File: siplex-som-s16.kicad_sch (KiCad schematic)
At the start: 1 part, among them J1 RFShield_OnePiece

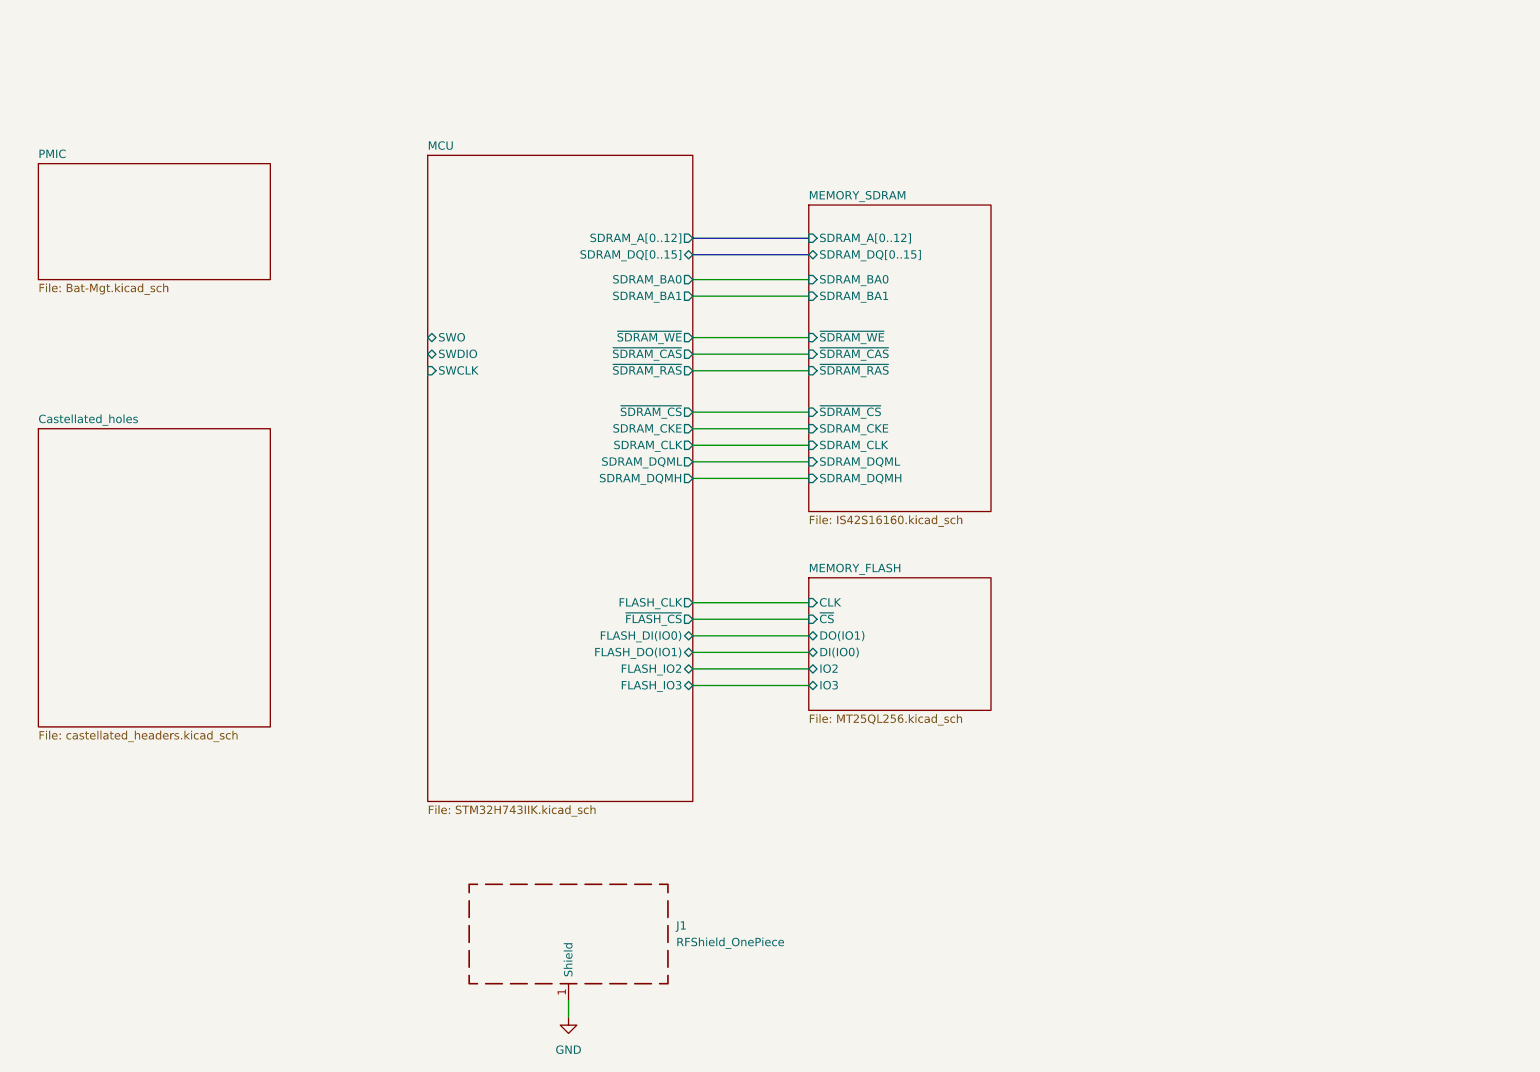
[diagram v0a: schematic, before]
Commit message: Add power
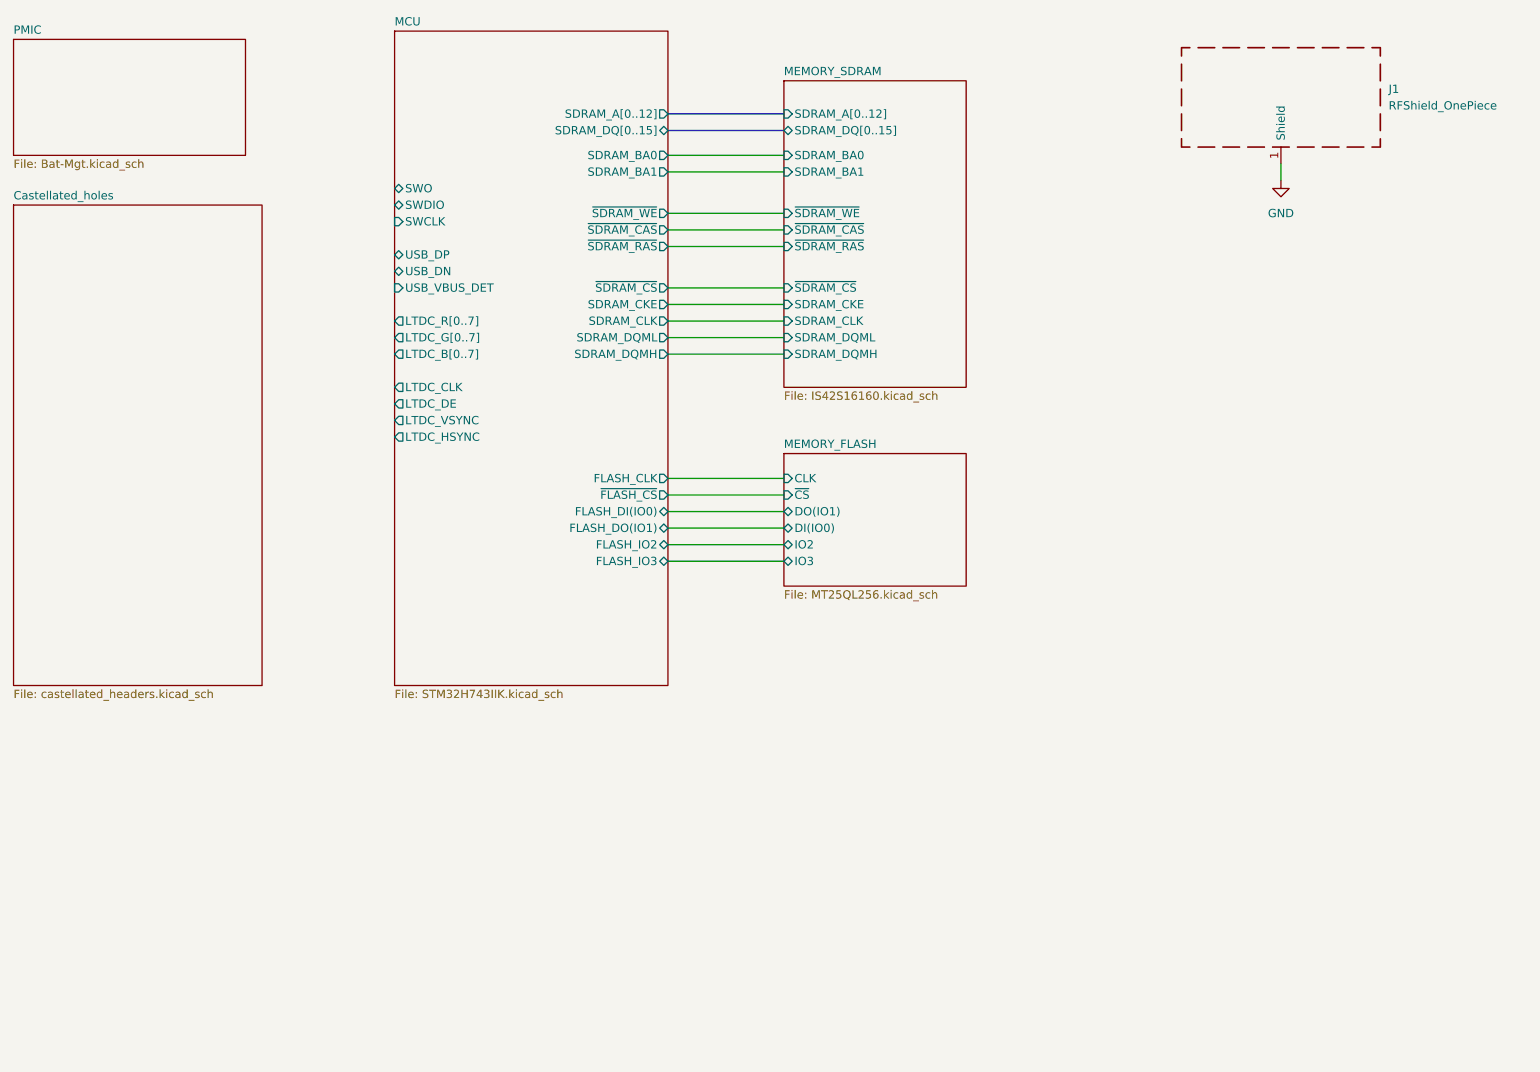
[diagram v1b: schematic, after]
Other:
- sheet MCU ports: added LTDC_B[0..7], LTDC_CLK, LTDC_DE, LTDC_G[0..7], LTDC_HSYNC, LTDC_R[0..7], LTDC_VSYNC, USB_DN, USB_DP, USB_VBUS_DET; removed none
- moved on the sheet: J1
